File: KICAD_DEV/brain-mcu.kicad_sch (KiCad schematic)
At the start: 22 parts, among them SW1 SW_Push, SW2 SW_Push, U1 STM32H743VITx, Y1 8 MHz, Y2 32.768 KHz

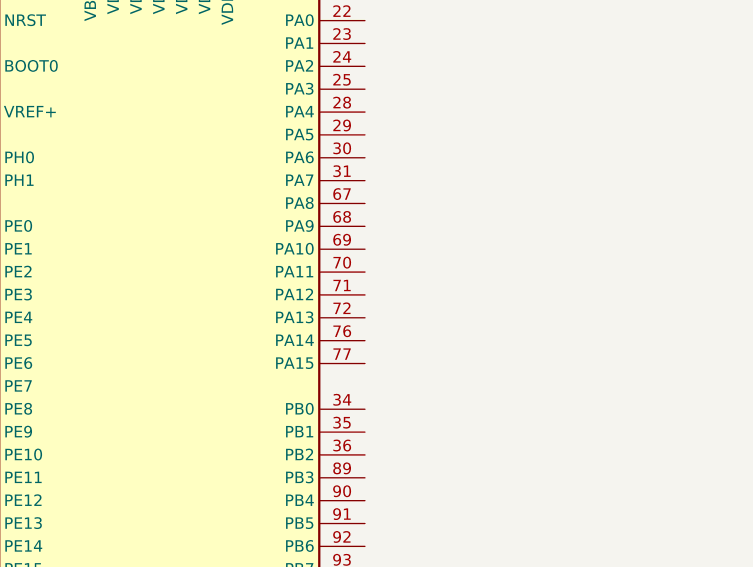
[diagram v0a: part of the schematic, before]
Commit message: forgot to wire USB data pairs, doing that now!
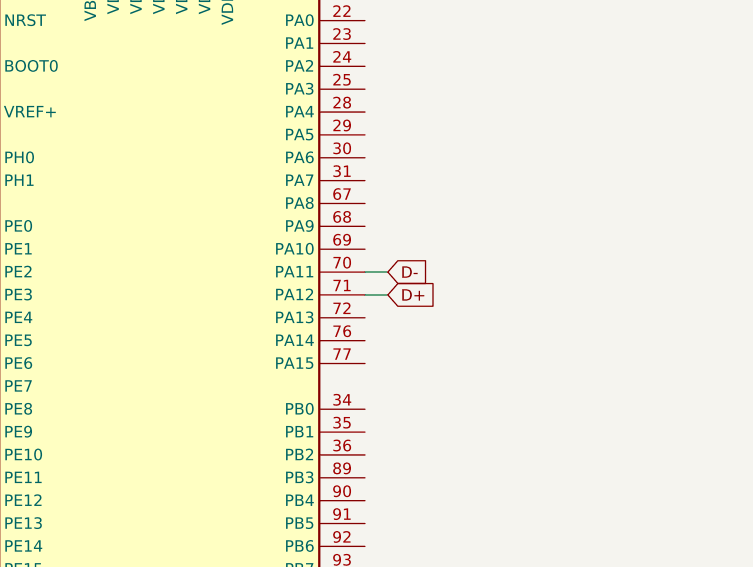
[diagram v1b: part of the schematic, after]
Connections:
- net D-: now reaches U1.70 (PA11)
- net D+: now reaches U1.71 (PA12)
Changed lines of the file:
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@@
+	(wire
+		(pts
+			(xy 247.65 128.27) (xy 245.11 128.27)
+		)
+		(stroke
+			(width 0)
+			(type default)
+		)
+	)
 	(wire
 		(pts
@@
 		(pts
 			(xy 76.2 148.59) (xy 76.2 147.32)
+		)
+		(stroke
+			(width 0)
+			(type default)
+		)
+	)
+	(wire
+		(pts
+			(xy 247.65 125.73) (xy 245.11 125.73)
 		)
 		(stroke
@@
 		)
 	)
+	(global_label "D-"
+		(shape input)
+		(at 247.65 125.73 0)
+		(fields_autoplaced yes)
+		(effects
+			(font
+				(size 1.27 1.27)
+			)
+			(justify left)
+		)
+		(property "Intersheetrefs" "${INTERSHEET_REFS}"
+			(at 253.4776 125.73 0)
+			(effects
+				(font
+					(size 1.27 1.27)
+				)
+				(justify left)
+				(hide yes)
+			)
+		)
+		(property "Netclass" "USB"
+			(at 247.65 127.9208 0)
+			(effects
+				(font
+					(size 1.27 1.27)
+				)
+				(justify left)
+				(hide yes)
+			)
+		)
+	)
 	(global_label "RESET"
 		(shape output)
@@
 			(effects
 				(font
+					(size 1.27 1.27)
+				)
+				(justify left)
+				(hide yes)
+			)
+		)
+	)
+	(global_label "D+"
+		(shape input)
+		(at 247.65 128.27 0)
+		(fields_autoplaced yes)
+		(effects
+			(font
+				(size 1.27 1.27)
+			)
+			(justify left)
+		)
+		(property "Intersheetrefs" "${INTERSHEET_REFS}"
+			(at 253.4776 128.27 0)
+			(effects
+				(font
+					(size 1.27 1.27)
+				)
+				(justify left)
+				(hide yes)
+			)
+		)
+		(property "Netclass" "USB"
+			(at 247.65 130.4608 0)
+			(effects
+				(font
